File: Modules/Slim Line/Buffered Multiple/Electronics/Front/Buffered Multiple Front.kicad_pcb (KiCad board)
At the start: 2 copper layers, 9.8 x 128.5 mm, 8 parts

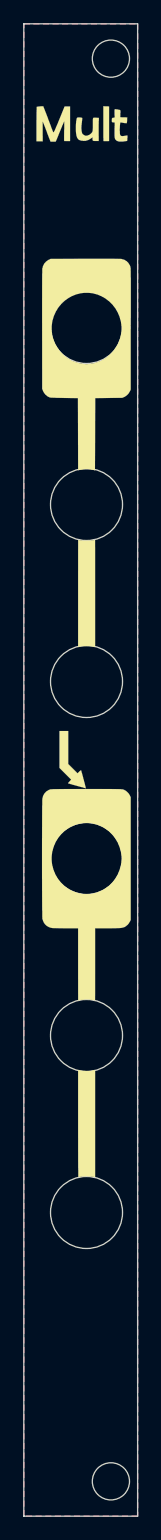
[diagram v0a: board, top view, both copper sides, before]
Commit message: Update
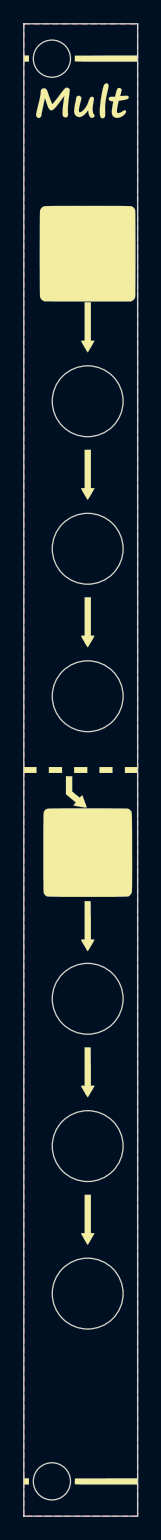
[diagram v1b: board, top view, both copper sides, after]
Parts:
- removed REF** (x6): Hole_D6.2mm, Front_Eurorack:Hole_D6.2mm
- removed REF**: Eurorack_2TE, Front_Eurorack:Eurorack_2TE
- added ?: , Bohrungen:Bohrung_6.1mm, F.Cu at (5.50, 109.3)
- added ?: , Bohrungen:Bohrung_3.2mm, F.Cu at (2.42, 3.00)
- added ?: , Bohrungen:Bohrung_6.1mm, F.Cu at (5.50, 96.6)
- added ?: , Bohrungen:Bohrung_6.1mm, F.Cu at (5.50, 84.0)
- added ?: , Bohrungen:Bohrung_6.1mm, F.Cu at (5.50, 71.4)
- added ?: , Bohrungen:Bohrung_6.1mm, F.Cu at (5.50, 57.9)
- added ?: , Bohrungen:Bohrung_6.1mm, F.Cu at (5.50, 45.2)
- added ?: , Bohrungen:Bohrung_6.1mm, F.Cu at (5.50, 32.5)
- added ?: , Bohrungen:Bohrung_6.1mm, F.Cu at (5.50, 19.8)
- added ?: , Bohrungen:Bohrung_3.2mm, F.Cu at (2.42, 125.5)
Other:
- board text added: "JLCJLCJLCJLC"
